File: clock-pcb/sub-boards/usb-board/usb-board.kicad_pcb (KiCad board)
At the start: 2 copper layers, 13.4 x 20 mm, 7 parts, among them J1 USB4145-03-0070-C, J8 Conn_01x04_Socket

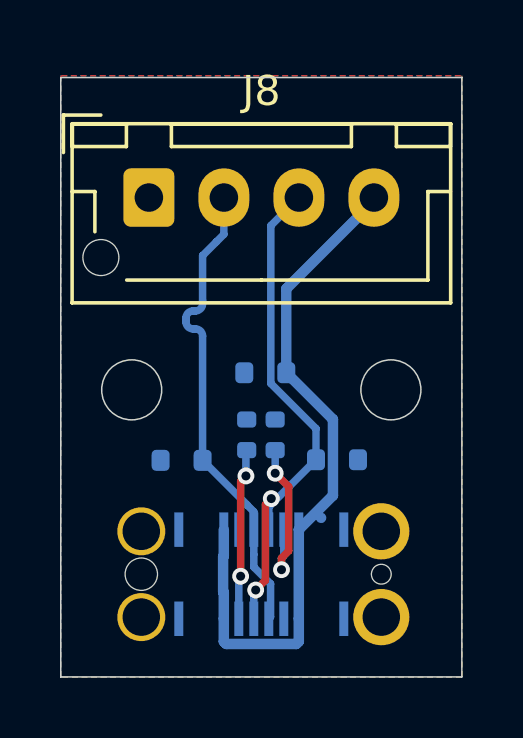
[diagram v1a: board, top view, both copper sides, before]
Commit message: panel
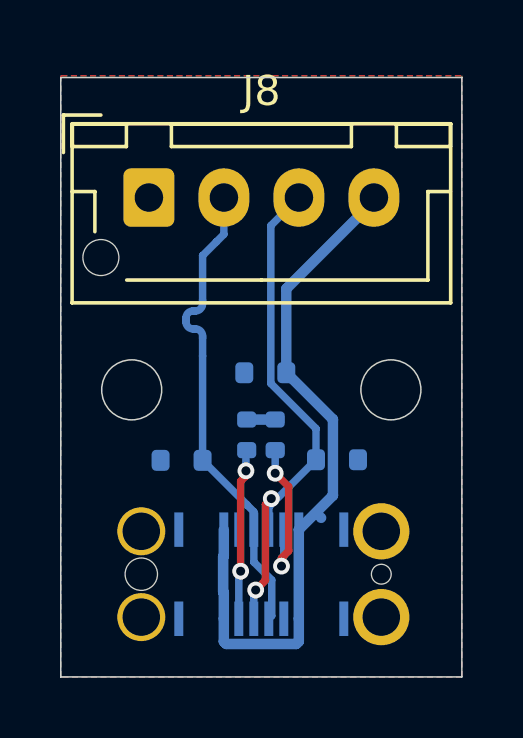
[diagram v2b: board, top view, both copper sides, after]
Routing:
- net GND: track 0.00 -> 0.95 mm
